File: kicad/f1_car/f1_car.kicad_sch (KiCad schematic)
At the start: 4 parts, among them U1 ESP32-C3-DevKitC-02

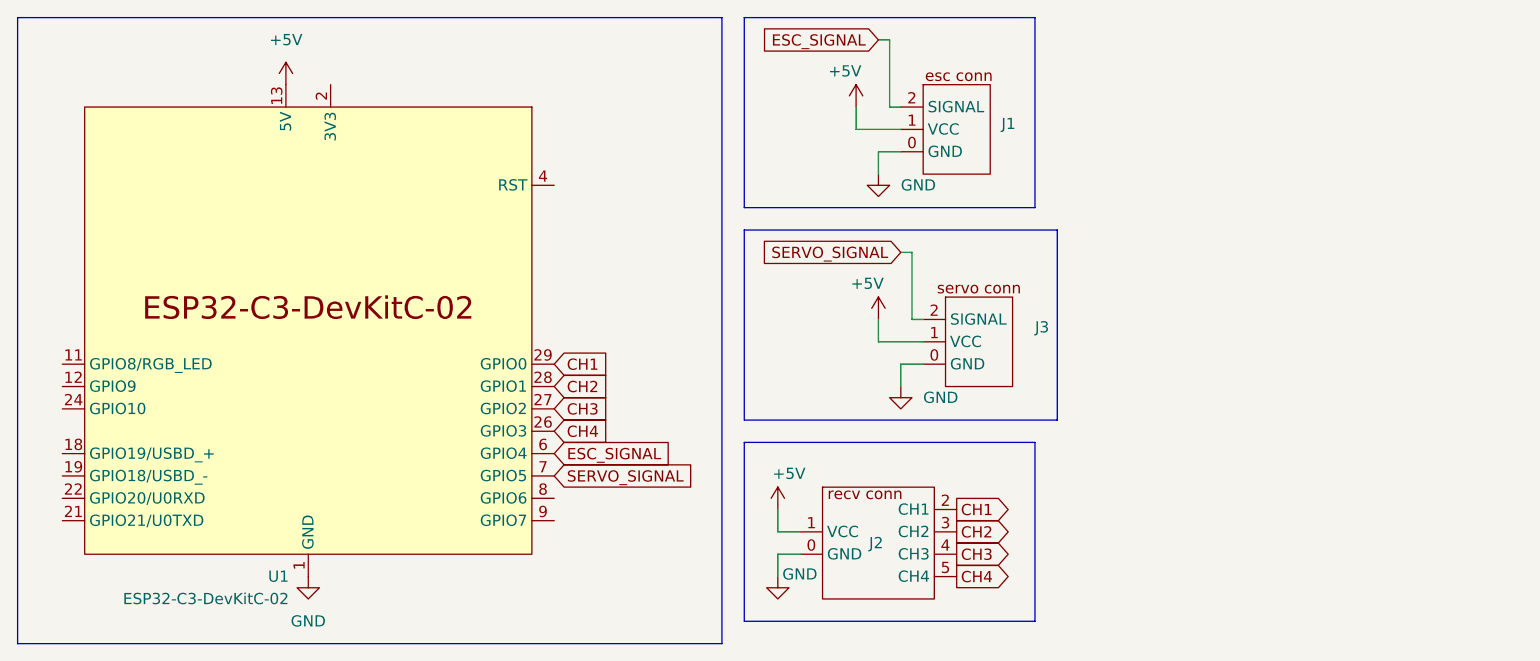
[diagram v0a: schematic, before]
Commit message: schematic pdf
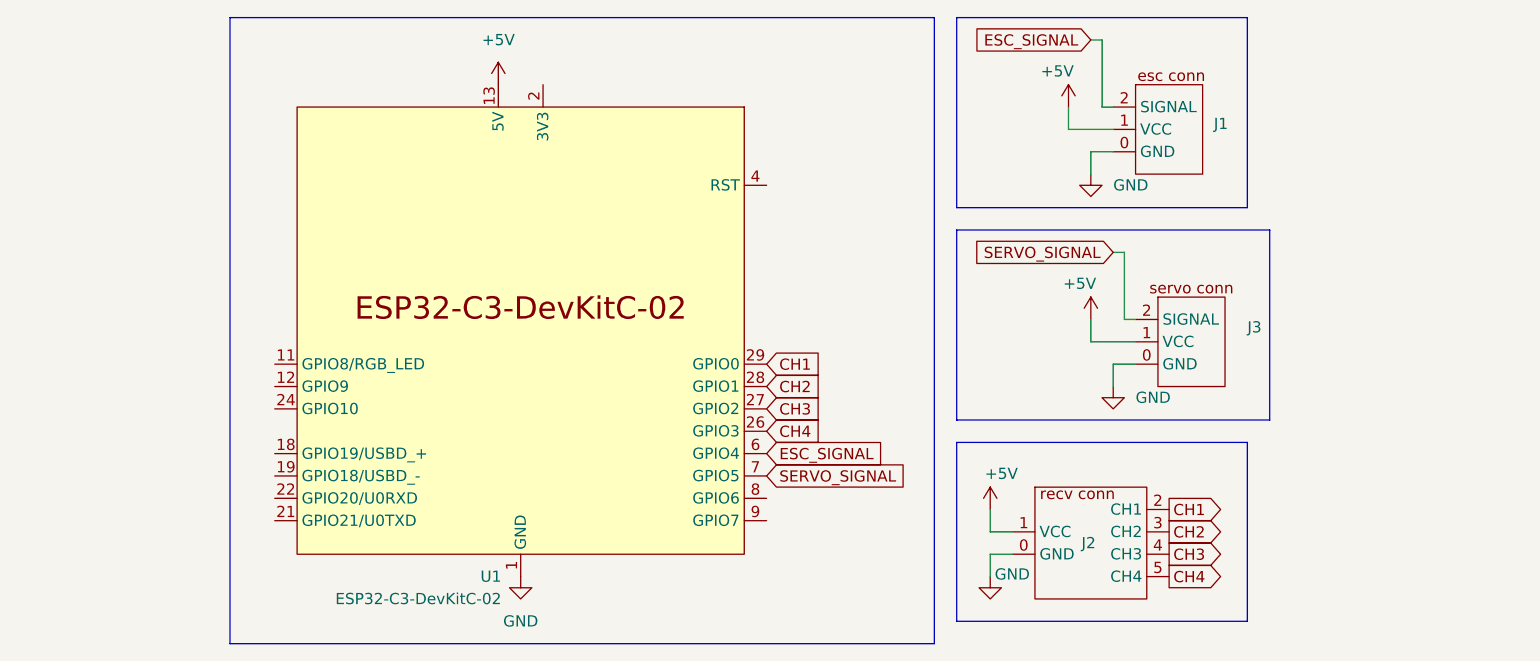
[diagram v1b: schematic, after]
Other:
- company: (none) -> ITIS E.MATTEI URBINO
- title: (none) -> F1 Car
- moved on the sheet: J1, J2, J3, U1

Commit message: pcb shield
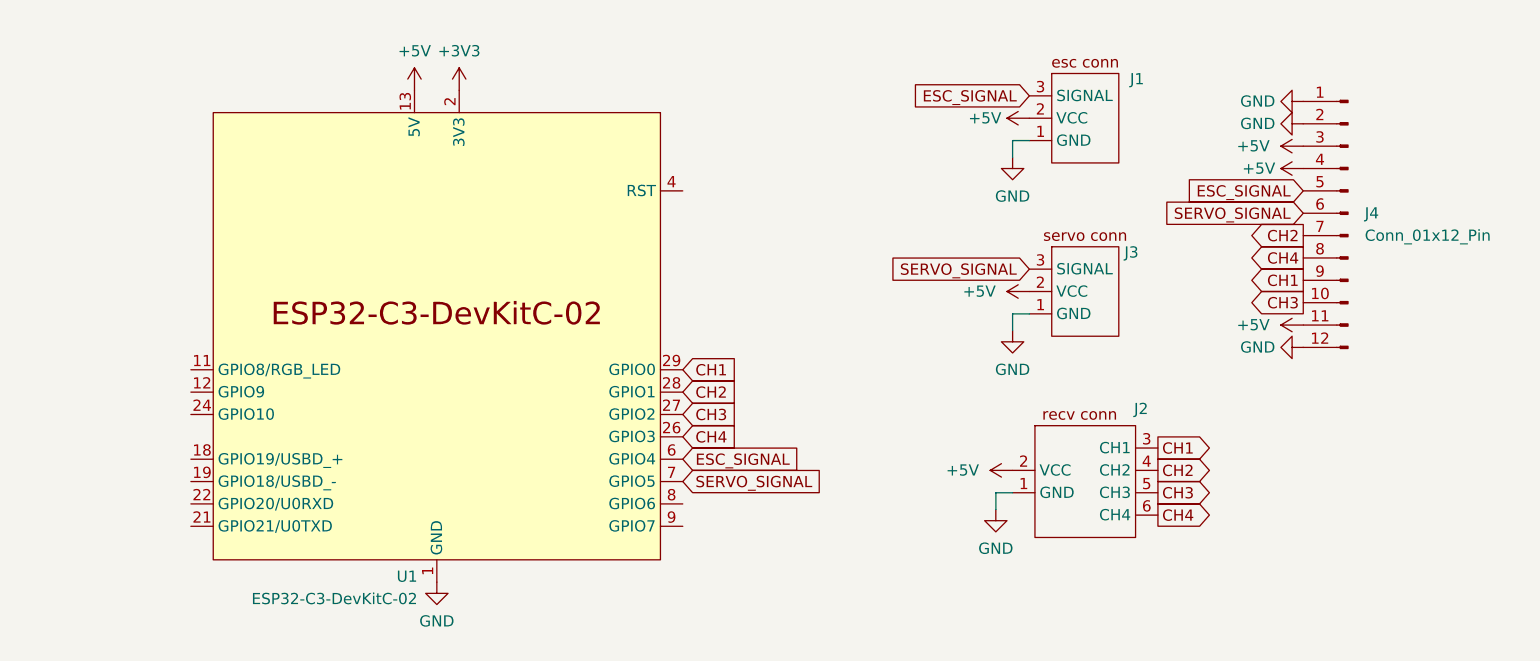
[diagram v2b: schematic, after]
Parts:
- removed J1: ~, symbol lib_progetto:esc_connector
- removed J2: ~, symbol lib_progetto:receiver_connector
- removed J3: ~, symbol lib_progetto:steering_servo_connector
- added J1: ~, symbol connettori_progetto:esc_conn
- added J2: ~, symbol connettori_progetto:recv_conn
- added J3: ~, symbol connettori_progetto:servo_conn
- added J4: Conn_01x12_Pin, Connector_PinHeader_2.54mm:PinHeader_2x06_P2.54mm_Horizontal, symbol Connector:Conn_01x12_Pin
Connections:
- net +5V: now also J1.2 (VCC), J2.2 (VCC), J3.2 (VCC), J4.11 (Pin_11), J4.3 (Pin_3), J4.4 (Pin_4)
- net CH1: now also J2.3 (CH1), J4.9 (Pin_9)
- net CH2: now also J2.4 (CH2), J4.7 (Pin_7)
- net CH3: now also J2.5 (CH3), J4.10 (Pin_10)
- net CH4: now also J2.6 (CH4), J4.8 (Pin_8)
- net ESC_SIGNAL: now also J1.3 (SIGNAL), J4.5 (Pin_5)
- net GND: now also J1.1 (GND), J2.1 (GND), J3.1 (GND), J4.1 (Pin_1), J4.12 (Pin_12), J4.2 (Pin_2)
- net SERVO_SIGNAL: now also J3.3 (SIGNAL), J4.6 (Pin_6)
- net 3V3 renamed +3V3
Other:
- company: ITIS E.MATTEI URBINO -> (none)
- title: F1 Car -> (none)
